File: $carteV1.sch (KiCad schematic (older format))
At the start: 53 parts, among them CON1 USB-MINI-B, J12 FILTER_IOUT_DUT2, J6 REF_CLK_DUT2, J7 CRYSTAL OUTDUT2, P2 CONN_2X2, P3 CONN_2, T4 BALUN, T8 T1-1T, U1 AD9954, U2 LM1117MP-1.8, U3 LM1117MP-1.8, U4 LM1117MP-3.3, U5 MCP2210-SO, X1 25mhz, X2 12mhz

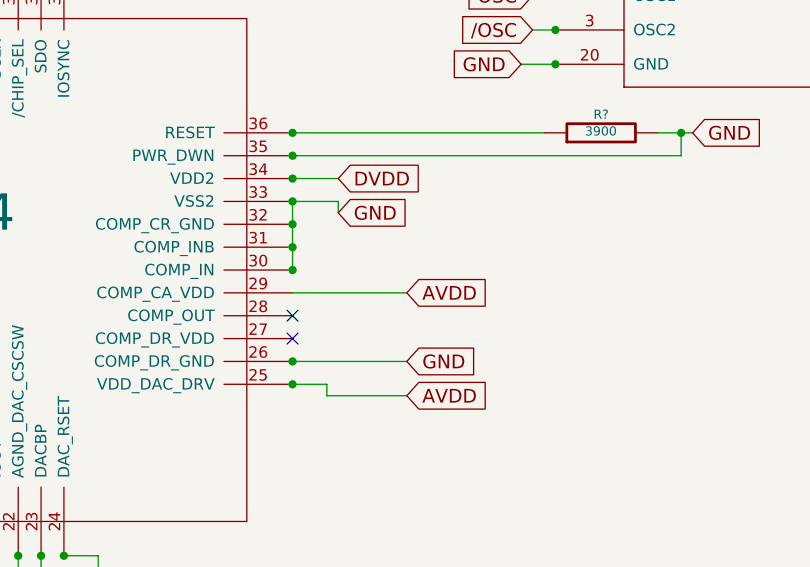
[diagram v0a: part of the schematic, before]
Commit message: modification ad9954
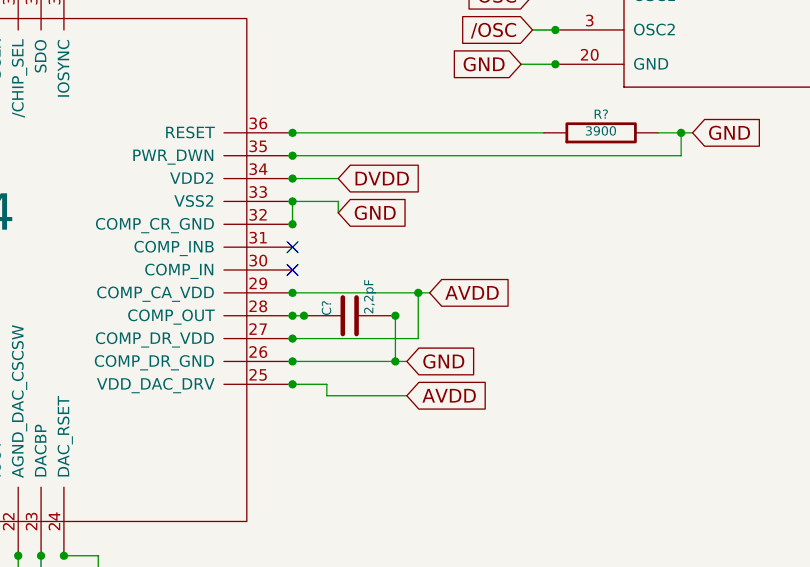
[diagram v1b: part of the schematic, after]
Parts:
- added C?: 2,2pF, ~, symbol C
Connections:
- net AVDD: now also U1.27 (COMP_DR_VDD)
- net GND: now also C?.2; no longer U1.30 (COMP_IN), U1.31 (COMP_INB)
- net at U1.28 (COMP_OUT): now also C?.1
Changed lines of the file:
@@
 Text GLabel 7400 2850 2    60   Input ~ 0
 GND
-Text GLabel 7700 3200 2    60   Input ~ 0
+Text GLabel 7800 3200 2    60   Input ~ 0
 AVDD
 Text GLabel 7700 3650 2    60   Input ~ 0
@@
 Text GLabel 7450 1450 2    60   Input ~ 0
 /OSC
-NoConn ~ 7200 3300
-NoConn ~ 7200 3400
 NoConn ~ 10050 1100
 NoConn ~ 10050 1200
@@
 Text GLabel 5200 1400 1    60   Input ~ 0
 GND
+NoConn ~ 5400 1750
+NoConn ~ 5500 1750
 Wire Wire Line
 	8250 2050 8350 2050
@@
 Connection ~ 7200 2700
 Wire Wire Line
-	7200 3200 7700 3200
-Wire Wire Line
 	7200 3600 7350 3600
 Wire Wire Line
@@
 	8800 2500 8950 2500
 Wire Wire Line
-	7200 2800 7200 3100
+	7200 2900 7200 2800
 Connection ~ 7200 2900
 Wire Wire Line
@@
 Connection ~ 5300 1750
 Connection ~ 6800 1500
-NoConn ~ 5400 1750
-NoConn ~ 5500 1750
 Wire Wire Line
 	6850 1750 6200 1750
@@
 Connection ~ 7200 2600
 Connection ~ 7200 2500
-Connection ~ 7200 3000
-Connection ~ 7200 3100
+NoConn ~ 7200 3000
+NoConn ~ 7200 3100
+$Comp
+L C C?
+U 1 1 538342CC
+P 7450 3300
+F 0 "C?" H 7450 3400 40  0000 L CNN
+F 1 "2,2pF" H 7456 3215 40  0000 L CNN
+F 2 "~" H 7488 3150 30  0000 C CNN
+F 3 "~" H 7450 3300 60  0000 C CNN
+	1    7450 3300
+	0    -1   -1   0
+$EndComp
+Wire Wire Line
+	7200 3300 7250 3300
+Wire Wire Line
+	7650 3300 7650 3500
+Connection ~ 7650 3500
+Wire Wire Line
+	7200 3200 7800 3200
+Wire Wire Line
+	7200 3400 7750 3400
+Wire Wire Line
+	7750 3400 7750 3200
+Connection ~ 7750 3200
+Connection ~ 7650 3300
+Connection ~ 7200 3300
+Connection ~ 7250 3300
+Connection ~ 7200 3200
+Connection ~ 7200 3400
 $EndSCHEMATC
